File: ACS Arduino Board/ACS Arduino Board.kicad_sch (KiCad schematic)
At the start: 11 parts, among them J1 TBLH10V-350-08BK, J2 TBLH10V-350-02BK, J3 TBLH10V-350-08BK, J4 TBLH10V-350-02BK, K1 CPC1706Y

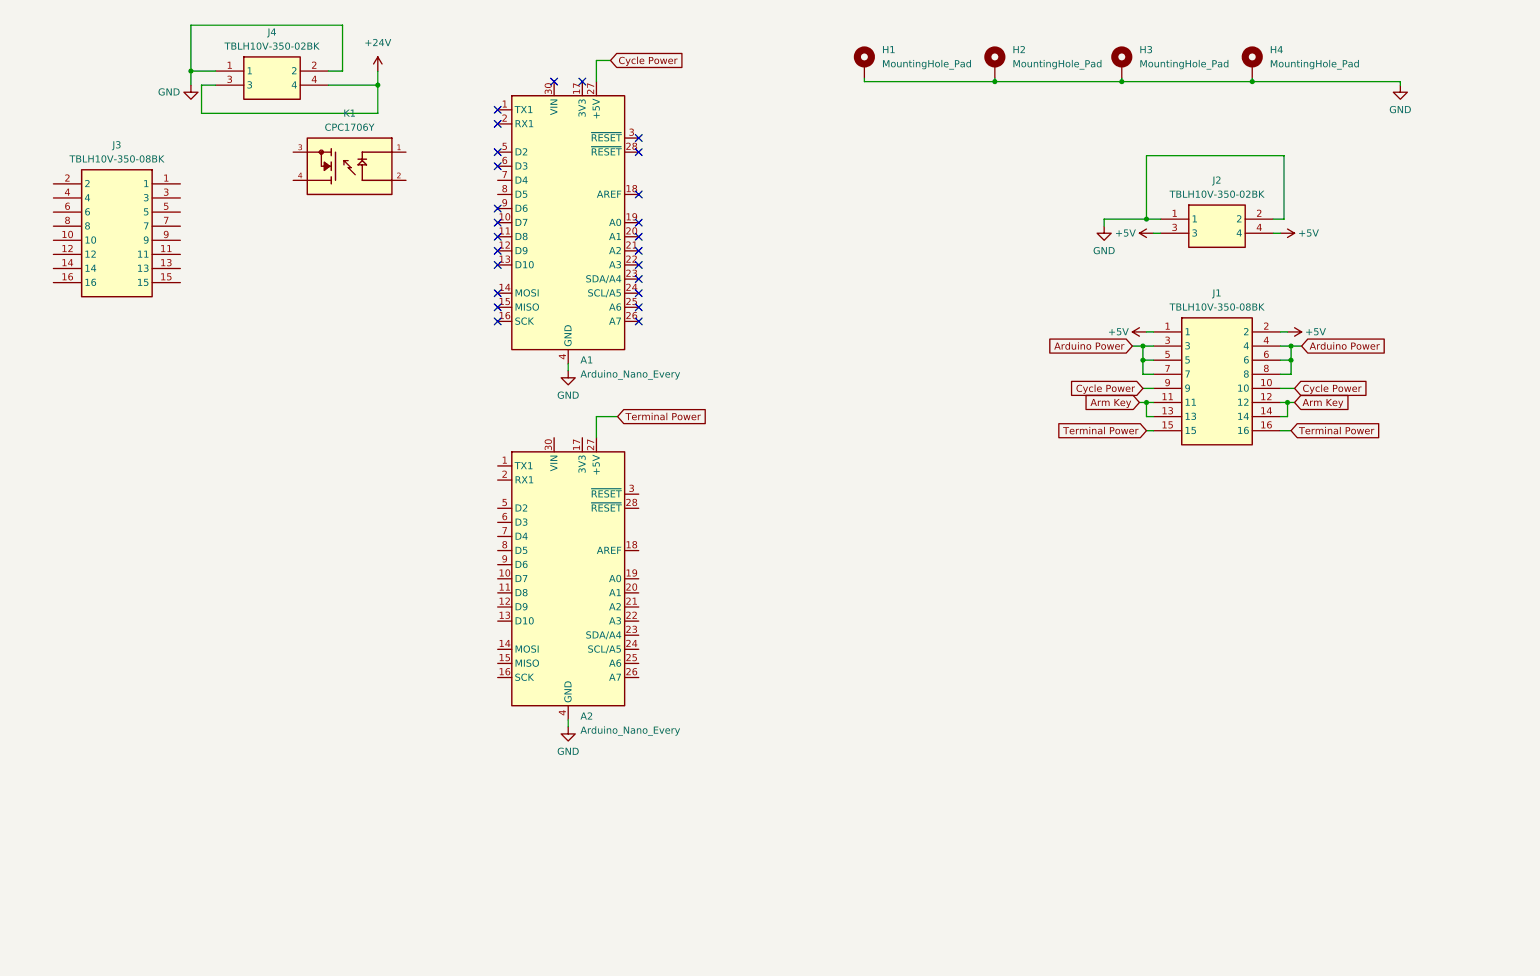
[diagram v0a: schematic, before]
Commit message: Lots of things
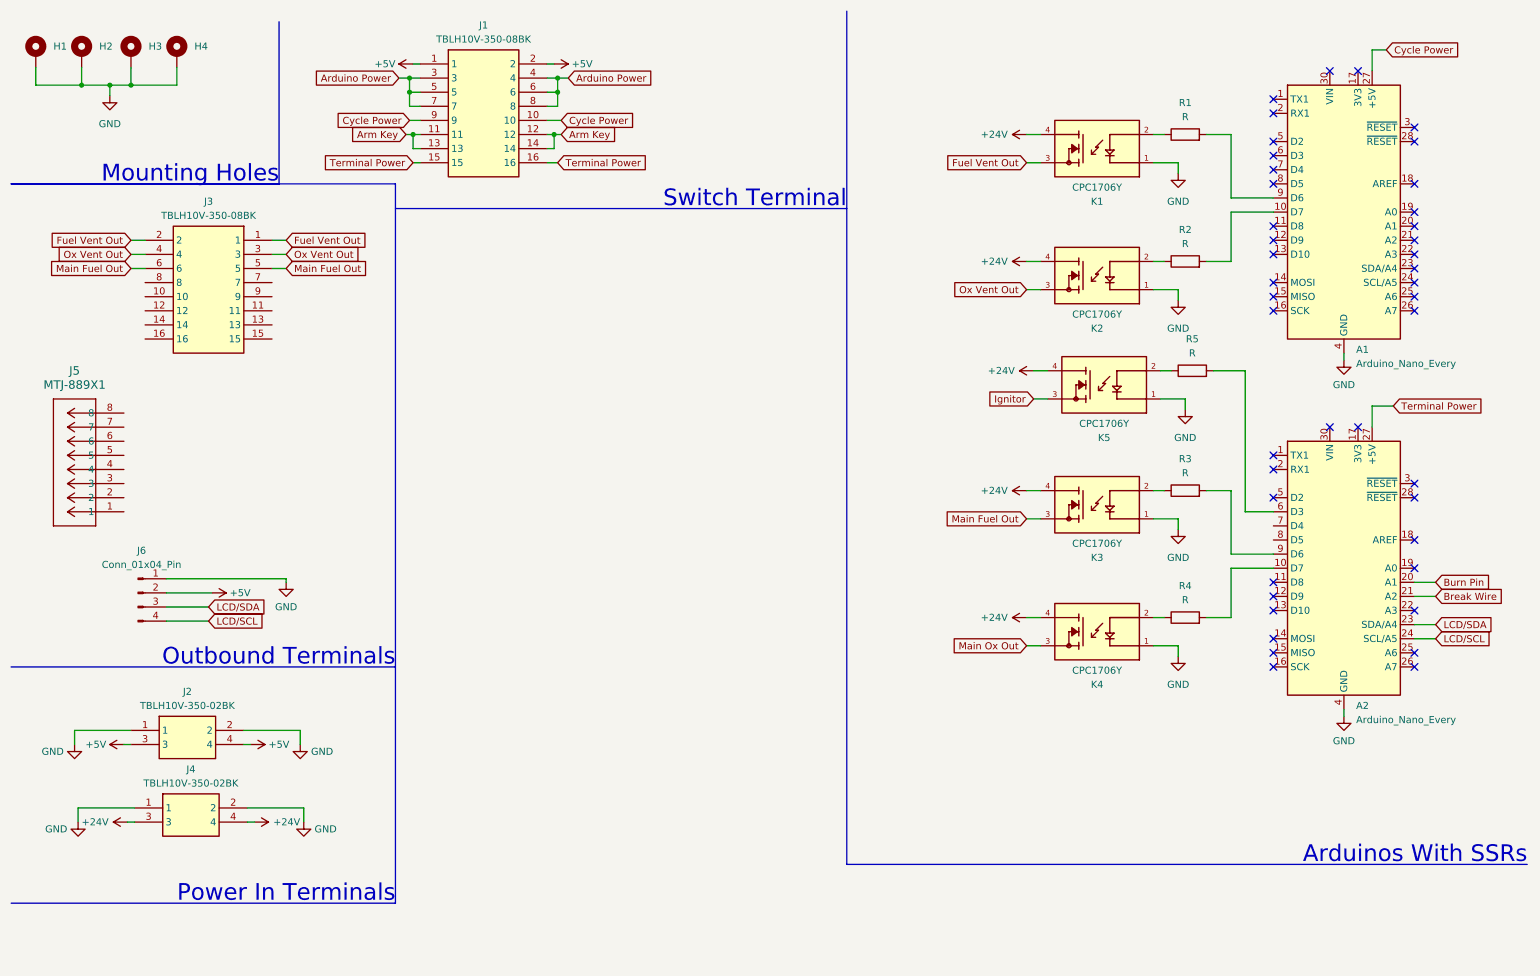
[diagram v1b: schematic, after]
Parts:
- added J5: MTJ-889X1, MTJ-889X1:CONN_MTJ-889X1_ADM, symbol MTJ-889X1:MTJ-889X1
- added J6: Conn_01x04_Pin, symbol Connector:Conn_01x04_Pin
- added K2, K3, K4, K5: CPC1706Y, CPC1706Y:RELAY_CPC1706Y, symbol CPC1706Y:CPC1706Y
- added R1, R2, R3, R4, R5: R, Resistor_THT:R_Axial_DIN0204_L3.6mm_D1.6mm_P5.08mm_Horizontal, symbol Device:R
- H1, H2, H3, H4: footprint (none) -> MountingHole:MountingHole_3.2mm_M3_DIN965_Pad_TopBottom
- J1, J3: footprint RHDR16W80P550X350_2X8_2870X850X1420P -> TBLH10V-350-08BK:RHDR16W80P550X350_2X8_2870X850X1420P
- J2, J4: footprint RHDR4W80P550X350_2X2_770X850X1420P -> TBLH10V-350-02BK:RHDR4W80P550X350_2X2_770X850X1420P
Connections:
- net +24V: now also K1.4, K2.4, K3.4, K4.4, K5.4
- net +5V: now also J6.2 (Pin_2)
- net GND: now also K1.1, J6.1 (Pin_1), K2.1, K3.1, K4.1, K5.1
- net at K1.2: now also R1.1
- net Fuel Vent Out: now reaches K1.3
- net Fuel Vent Out: now also J3.1, J3.2
- net at A2.10 (D7): now also R4.2
- net Burn Pin: now reaches A2.20 (A1)
- net Break Wire: now reaches A2.21 (A2)
- net LCD/SDA: now reaches A2.23 (SDA/A4)
- net LCD/SDA: now also J6.3 (Pin_3)
- net LCD/SCL: now reaches A2.24 (SCL/A5)
- net LCD/SCL: now also J6.4 (Pin_4)
- net at A2.6 (D3): now also R5.2
- net at A2.9 (D6): now also R3.2
- net at A1.10 (D7): now also R2.2
- net at A1.9 (D6): now also R1.2
- net Ox Vent Out: now reaches J3.3
- net Ox Vent Out: now also J3.4, K2.3
- net Main Fuel Out: now reaches J3.5
- net Main Fuel Out: now also J3.6, K3.3
- new net: K3.2, R3.1
- new net: K4.2, R4.1
- new net: K5.2, R5.1
- new net: K2.2, R2.1
- new net Ignitor: K5.3
- new net Main Ox Out: K4.3
- no-connect marks 25 -> 43
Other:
- note added: "Arduinos With SSRs"
- note added: "Mounting Holes"
- note added: "Outbound Terminals"
- note added: "Power In Terminals"
- note added: "Switch Terminal"
- moved on the sheet: A1, A2, J1, J2, J3, J4, K1

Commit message: Piss
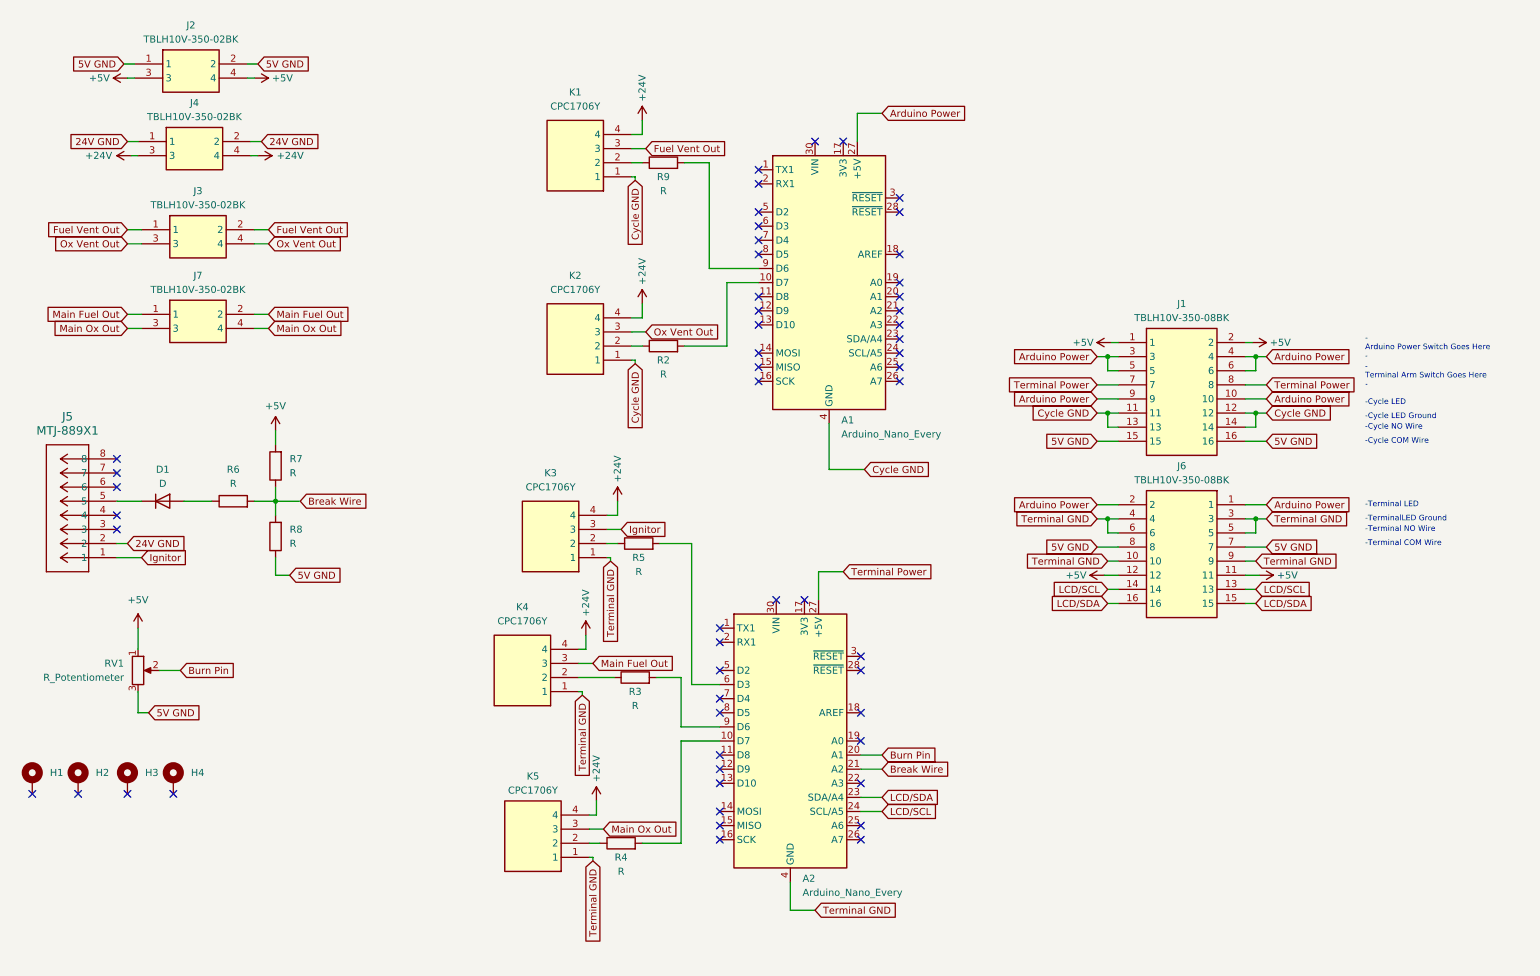
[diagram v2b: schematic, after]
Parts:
- removed J3: TBLH10V-350-08BK, TBLH10V-350-08BK:RHDR16W80P550X350_2X8_2870X850X1420P, symbol TBLH10V-350-08BK:TBLH10V-350-08BK
- removed J6: Conn_01x04_Pin, symbol Connector:Conn_01x04_Pin
- removed R1: R, Resistor_THT:R_Axial_DIN0204_L3.6mm_D1.6mm_P5.08mm_Horizontal, symbol Device:R
- added D1: D, Diode_THT:D_A-405_P7.62mm_Horizontal, symbol Device:D
- added J3, J7: TBLH10V-350-02BK, TBLH10V-350-02BK:RHDR4W80P550X350_2X2_770X850X1420P, symbol TBLH10V-350-02BK:TBLH10V-350-02BK
- added J6: TBLH10V-350-08BK, TBLH10V-350-08BK:RHDR16W80P550X350_2X8_2870X850X1420P, symbol TBLH10V-350-08BK:TBLH10V-350-08BK
- added R6, R7, R8, R9: R, Resistor_THT:R_Axial_DIN0204_L3.6mm_D1.6mm_P5.08mm_Horizontal, symbol Device:R
- added RV1: R_Potentiometer, Connector_PinSocket_2.54mm:PinSocket_1x03_P2.54mm_Vertical, symbol Device:R_Potentiometer
- K1, K2, K3, K4, K5: footprint CPC1706Y:RELAY_CPC1706Y -> RelayCPC:CPC1706Y; MANUFACTURER IXYS -> (none); Manufacturer_Name (none) -> LITTELFUSE; Manufacturer_Part_Number (none) -> CPC1706Y; Mouser Part Number (none) -> 849-CPC1706Y; Mouser Price/Stock (none) -> https://www.mouser.co.uk/ProductDetail/IXYS-Integrated-Circ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; STANDARD Manufacturer Recommendations -> (none)
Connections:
- net Cycle Power is gone; now on net Arduino Power: A1.27 (+5V), J1.10, J1.9
- net +5V: now also J6.11, J6.12, R7.2, RV1.1
- net Arduino Power: now also J6.1, J6.2; no longer J1.7, J1.8
- net Break Wire: now also R6.2, R7.1, R8.2
- net Burn Pin: now also RV1.2
- net Fuel Vent Out: now also J3.1, J3.2
- net Ignitor: now also J5.1, K3.3; no longer K5.3
- net LCD/SCL: now also J6.13, J6.14
- net LCD/SDA: now also J6.15, J6.16
- net Main Fuel Out: now also K4.3, J7.1, J7.2; no longer K3.3
- net Main Ox Out: now also K5.3, J7.3, J7.4; no longer K4.3
- net Ox Vent Out: now also J3.3, J3.4
- net Terminal Power: now also J1.7, J1.8; no longer J1.15, J1.16
- net at R3.1: now also K4.2; no longer K3.2
- net at R4.1: now also K5.2; no longer K4.2
- net at R5.1: now also K3.2; no longer K5.2
- net 24V GND: now reaches J5.2
- net 24V GND: now also J4.1, J4.2
- net at J5.5: now also D1.1 (K)
- net at K1.2: now also R9.1
- net at A1.9 (D6): now also R9.2
- net Arm Key renamed Cycle GND
- net Cycle GND: now also A1.29 (GND), A1.4 (GND), K1.1, K2.1
- removed net GND: A1.29 (GND), A1.4 (GND), A2.29 (GND), A2.4 (GND), H1.1, H2.1, H3.1, H4.1, J2.1, J2.2, J4.1, J4.2, K1.1, K2.1, K3.1, K4.1, K5.1
- new net: D1.2 (A), R6.1
- new net 5V GND: J1.15, J1.16, J2.1, J2.2, J6.7, J6.8, R8.1, RV1.3
- new net Terminal GND: A2.29 (GND), A2.4 (GND), J6.10, J6.3, J6.4, J6.5, J6.6, J6.9, K3.1, K4.1, K5.1
- no-connect marks 43 -> 54
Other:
- note added: "- Arduino Power Switch Goes Here -"
- note added: "- Terminal Arm Switch Goes Here -"
- note added: "-Cycle COM Wire"
- note added: "-Cycle LED"
- note added: "-Cycle LED Ground"
- note added: "-Cycle NO Wire"
- note added: "-Terminal COM Wire"
- note added: "-Terminal LED"
- note added: "-Terminal NO Wire"
- note added: "-TerminalLED Ground"
- note removed: "Arduinos With SSRs"
- note removed: "Mounting Holes"
- note removed: "Outbound Terminals"
- note removed: "Power In Terminals"
- note removed: "Switch Terminal"
- moved on the sheet: A1, A2, H1, H2, H3, H4, J1, J2, J4, J5, R2, R3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
